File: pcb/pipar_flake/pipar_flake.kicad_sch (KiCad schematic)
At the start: 22 parts, among them SW2 SW_Wuerth_450301014042, U2 nice_nano

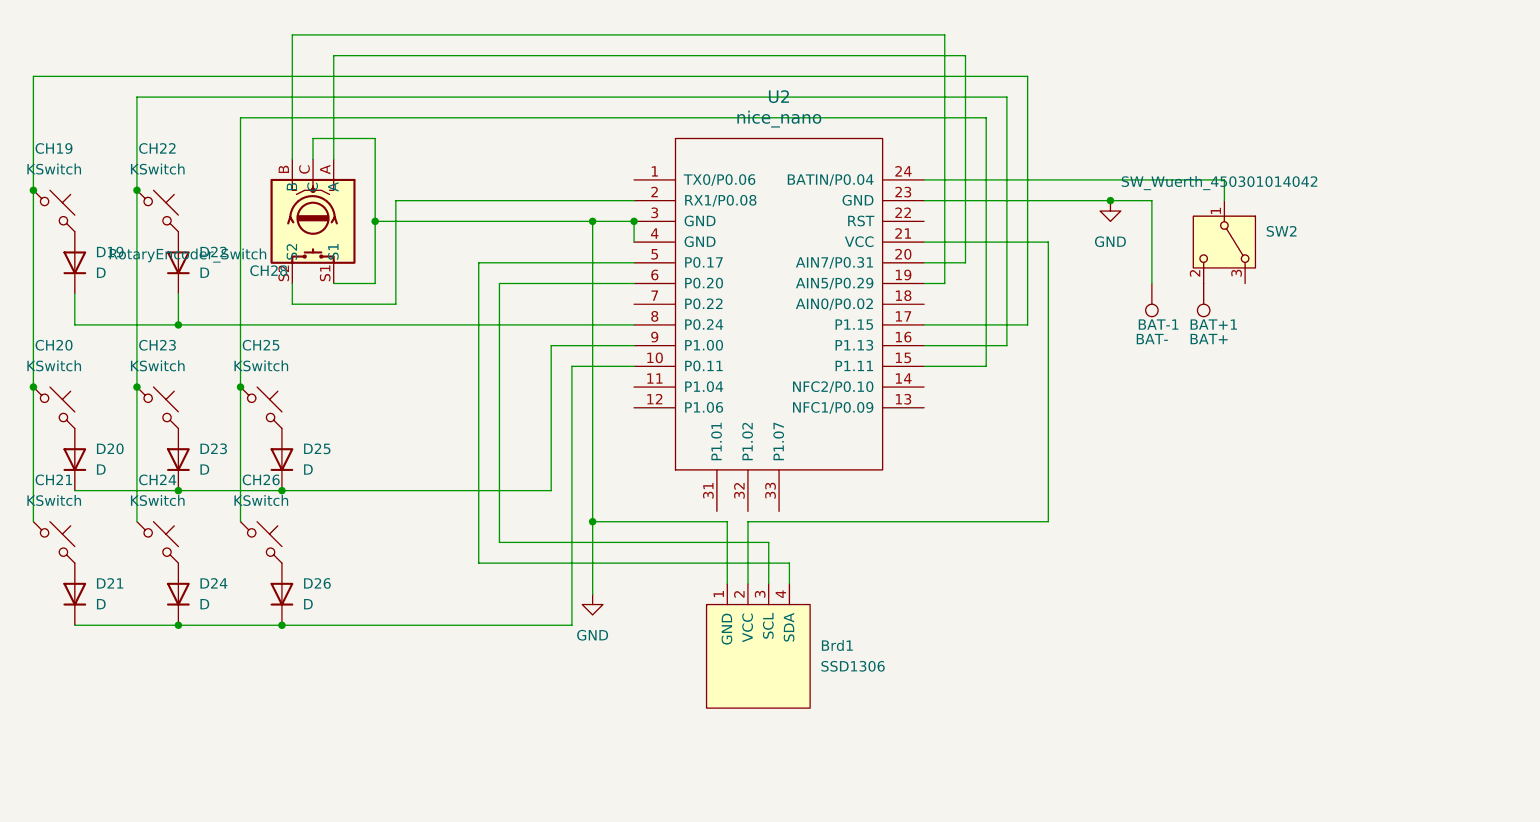
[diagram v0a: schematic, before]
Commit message: Reworks Pipar Flake to add LEDs and a bigger place for battery
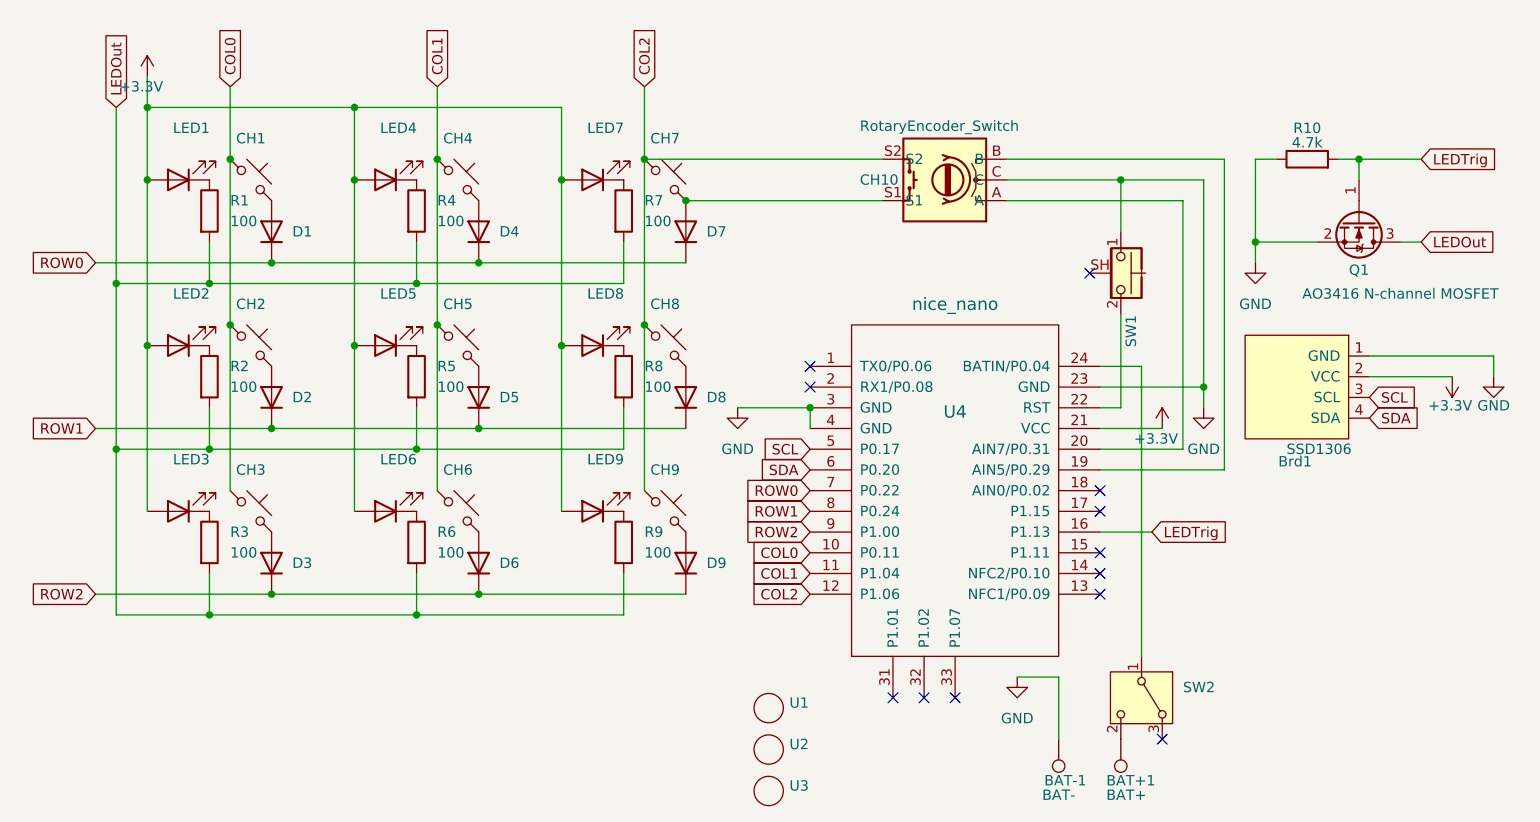
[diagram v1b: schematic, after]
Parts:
- removed CH19, CH20, CH21, CH22, CH23, CH24, CH25, CH26: KSwitch, keyswitches:Kailh_socket_PG1350_reversible, symbol marbastlib-choc:choc_v1_SW_HS_CPG135001S30
- removed CH28: RotaryEncoder_Switch, Rotary_Encoder:RotaryEncoder_Bourns_Vertical_PEL11L-4xxxF-Sxxxx_1, symbol Device:RotaryEncoder_Switch
- removed D19, D20, D21, D22, D23, D24, D25, D26: D, Diode_SMD:Nexperia_CFP3_SOD-123W, symbol Device:D
- removed U2: nice_nano, nice-nano-kicad:nice_nano, symbol nice_nano:nice_nano
- added CH1, CH2, CH3, CH4, CH5, CH6, CH8, CH9: KSwitch, yes:SW_Hotswap_Kailh_Choc_V1V2_LED_1.00u, symbol marbastlib-choc:choc_v1_SW_HS_CPG135001S30
- added CH10: RotaryEncoder_Switch, Rotary_Encoder:RotaryEncoder_Bourns_Vertical_PEL11L-4xxxF-Sxxxx_1, symbol Device:RotaryEncoder_Switch
- added CH7: KSwitch, PCM_Switch_Keyboard_Kailh:SW_Kailh_Choc_V1V2_1.00u, symbol marbastlib-choc:choc_v1_SW_HS_CPG135001S30
- added D1, D2, D3, D4, D5, D6, D7, D8, D9: D, Diode_SMD:Nexperia_CFP3_SOD-123W, symbol Device:D
- added LED1, LED2, LED3, LED4, LED5, LED6, LED7, LED8, LED9: ~, LED_SMD:LED_0805_2012Metric, symbol LED:IR26-21C_L110_TR8
- added Q1: AO3416 N-channel MOSFET, Package_TO_SOT_SMD:SOT-23, symbol Device:Q_NMOS_GSD
- added R1, R2, R3, R4, R5, R6, R7, R8, R9: 100, Resistor_SMD:R_0805_2012Metric, symbol Device:R
- added R10: 4.7k, Resistor_SMD:R_0805_2012Metric, symbol PCM_4ms_Resistor:10m_1206_250mW
- added SW1: CK_KMS2xxG, Button_Switch_SMD:SW_SPST_CK_KMS2xxGP, symbol Switch:CK_KMS2xxG
- added U1: ~, salt:Salt-smallest, symbol Trackpoint:Solder_Nut
- added U2, U3: ~, MountingHole:MountingHole_2.2mm_M2, symbol Trackpoint:Solder_Nut
- added U4: nice_nano, nice-nano-kicad:nice_nano, symbol nice_nano:nice_nano
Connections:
- net GND: now also CH10.C, Q1.2 (S), R10.1, SW1.1, U4.23 (GND), U4.3 (GND), U4.4 (GND)
- net +3.3V: now reaches Brd1.2 (VCC)
- net +3.3V: now also LED1.2 (A), LED2.2 (A), LED3.2 (A), LED4.2 (A), LED5.2 (A), LED6.2 (A), LED7.2 (A), LED8.2 (A), LED9.2 (A), U4.21 (VCC)
- net SCL: now reaches Brd1.3 (SCL)
- net SCL: now also U4.5 (P0.17)
- net SDA: now reaches Brd1.4 (SDA)
- net SDA: now also U4.6 (P0.20)
- net at SW2.1 (B): now also U4.24 (BATIN/P0.04)
- new net: CH4.2, D4.2 (A)
- new net: LED3.1 (K), R3.1
- new net: LED7.1 (K), R7.1
- new net: CH10.A, U4.20 (AIN7/P0.31)
- new net: CH10.B, U4.19 (AIN5/P0.29)
- new net: CH10.S1, CH7.2, D7.2 (A)
- new net: SW1.2, U4.22 (RST)
- new net: LED4.1 (K), R4.1
- new net: CH6.2, D6.2 (A)
- new net: CH5.2, D5.2 (A)
- new net: LED9.1 (K), R9.1
- new net: CH8.2, D8.2 (A)
- new net: CH3.2, D3.2 (A)
- new net: LED2.1 (K), R2.1
- new net: LED5.1 (K), R5.1
- new net: LED1.1 (K), R1.1
- new net: CH1.2, D1.2 (A)
- new net: LED8.1 (K), R8.1
- new net: CH9.2, D9.2 (A)
- new net: CH2.2, D2.2 (A)
- new net: LED6.1 (K), R6.1
- new net COL0: CH1.1, CH2.1, CH3.1, U4.10 (P0.11)
- new net COL1: CH4.1, CH5.1, CH6.1, U4.11 (P1.04)
- new net COL2: CH10.S2, CH7.1, CH8.1, CH9.1, U4.12 (P1.06)
- new net LEDOut: Q1.3 (D), R1.2, R2.2, R3.2, R4.2, R5.2, R6.2, R7.2, R8.2, R9.2
- new net LEDTrig: Q1.1 (G), R10.2, U4.16 (P1.13)
- new net ROW0: D1.1 (K), D4.1 (K), D7.1 (K), U4.7 (P0.22)
- new net ROW1: D2.1 (K), D5.1 (K), D8.1 (K), U4.8 (P0.24)
- new net ROW2: D3.1 (K), D6.1 (K), D9.1 (K), U4.9 (P1.00)
- no-connect marks 0 -> 12

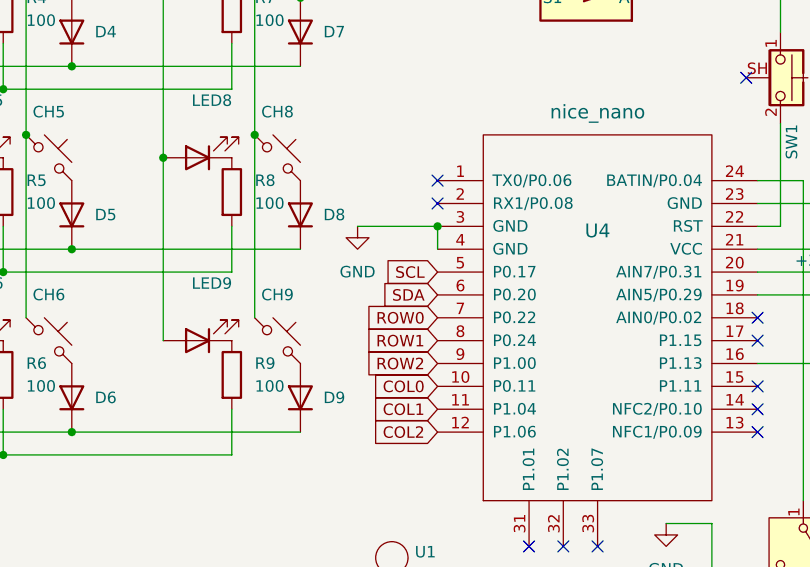
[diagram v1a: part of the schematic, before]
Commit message: swap sda and scl pins
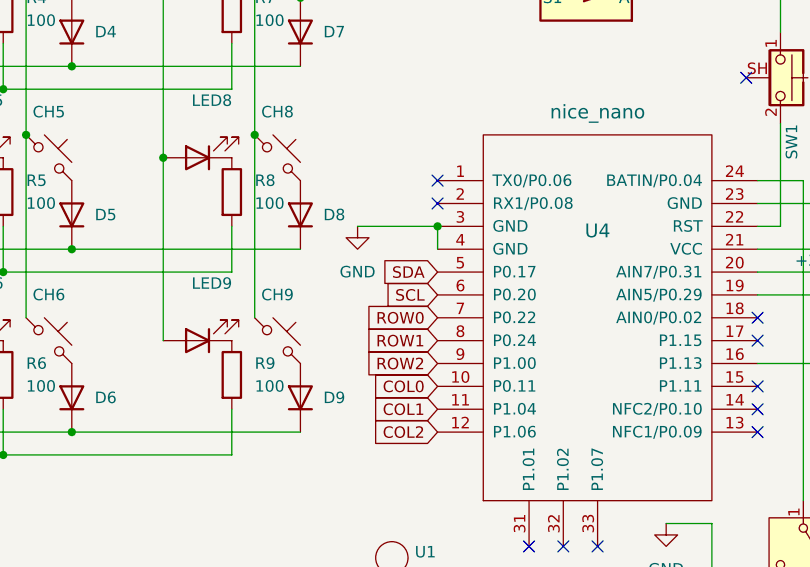
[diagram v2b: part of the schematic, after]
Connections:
- net SCL: now also U4.6 (P0.20); no longer U4.5 (P0.17)
- net SDA: now also U4.5 (P0.17); no longer U4.6 (P0.20)
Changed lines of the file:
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@@
+		)
+	)
+	(global_label "SDA"
+		(shape input)
+		(at 109.22 64.77 180)
+		(fields_autoplaced yes)
+		(effects
+			(font
+				(size 1.27 1.27)
+			)
+			(justify right)
+		)
+		(property "Intersheetrefs" "${INTERSHEET_REFS}"
+			(at 102.6667 64.77 0)
+			(effects
+				(font
+					(size 1.27 1.27)
+				)
+				(justify right)
+				(hide yes)
+			)
 		)
 	)
 	(global_label "SCL"
 		(shape input)
-		(at 109.22 64.77 180)
-		(fields_autoplaced yes)
-		(effects
-			(font
-				(size 1.27 1.27)
-			)
-			(justify right)
-		)
-		(property "Intersheetrefs" "${INTERSHEET_REFS}"
-			(at 102.7272 64.77 0)
+		(at 109.22 67.31 180)
+		(fields_autoplaced yes)
+		(effects
+			(font
+				(size 1.27 1.27)
+			)
+			(justify right)
+		)
+		(property "Intersheetrefs" "${INTERSHEET_REFS}"
+			(at 102.7272 67.31 0)
 			(effects
 				(font
@@
 			(effects
 				(font
-					(size 1.27 1.27)
-				)
-				(justify right)
-				(hide yes)
-			)
-		)
-	)
-	(global_label "SDA"
-		(shape input)
-		(at 109.22 67.31 180)
-		(fields_autoplaced yes)
-		(effects
-			(font
-				(size 1.27 1.27)
-			)
-			(justify right)
-		)
-		(property "Intersheetrefs" "${INTERSHEET_REFS}"
-			(at 102.6667 67.31 0)
-			(effects
-				(font
